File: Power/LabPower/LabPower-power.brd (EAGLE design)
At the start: 97.8 x 128.9 mm, 60 parts, among them IC1 TNY264PN, Q1 STP11NM60ND, Q2 STP11NM60ND, T1 GDT_20X6.5, X1 MKDSN1,5/3-5,08, X2 MKDSN1,5/3-5,08

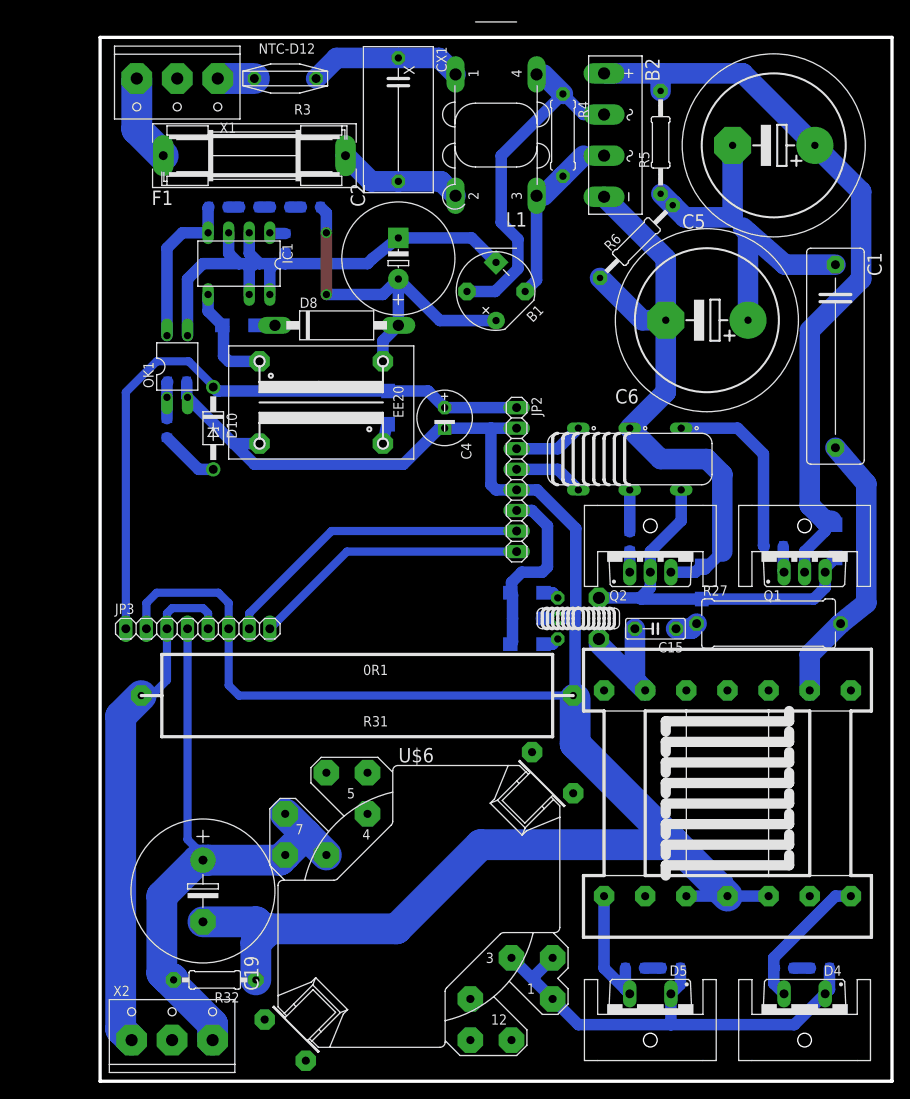
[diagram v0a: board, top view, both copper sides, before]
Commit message: _+
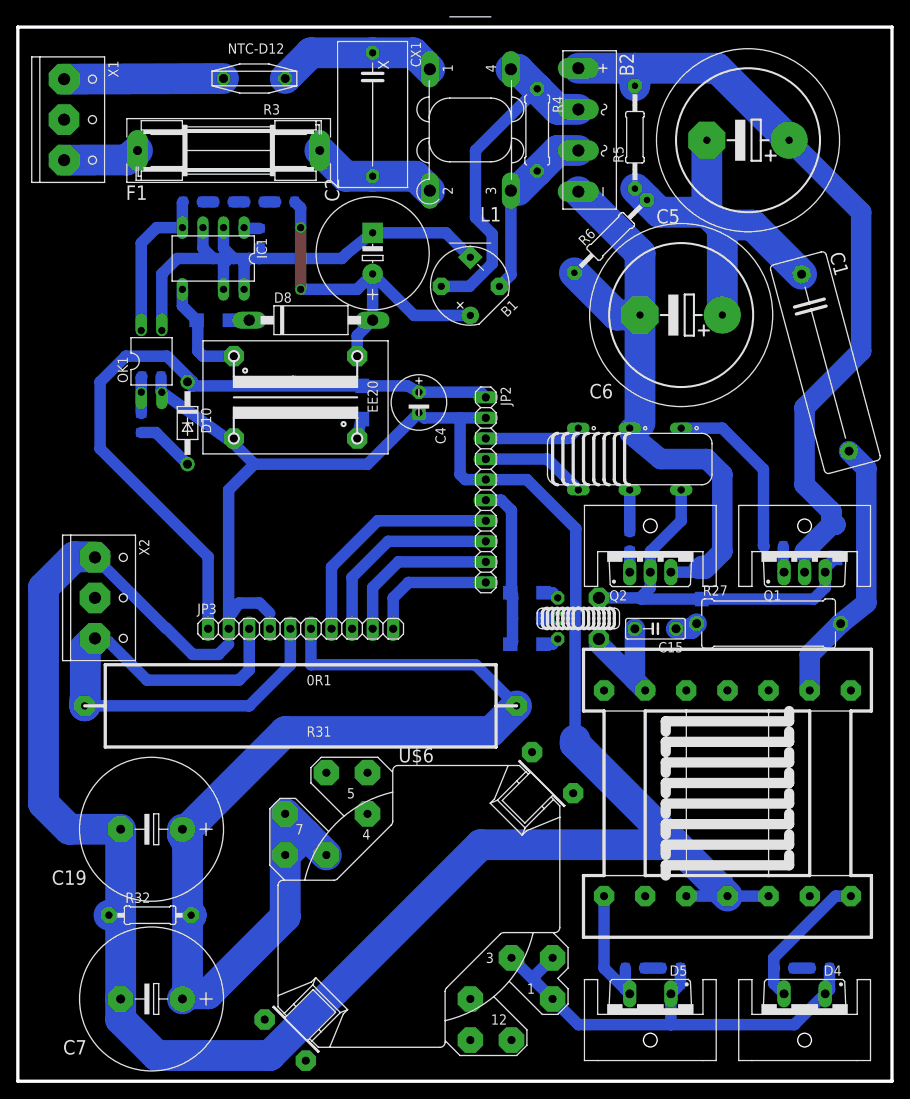
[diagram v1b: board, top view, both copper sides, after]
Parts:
- added C7: 2700u 63V, rcl:E7,5-18
- JP2, JP3: device pinhead:1X08 -> pinhead:1X10
- moved X2 55.4 mm to (-98.4, -69.8), turned to 270 degrees
- moved X1 14.9 mm to (-102.2, -10.8), turned to 270 degrees
- moved JP3 12.7 mm to (-73.0, -73.7)
- moved R32 11.3 mm to (-91.6, -109.0), turned to 0 degrees
- moved C19 9.92 mm to (-91.4, -98.4), turned to 180 degrees
- moved R31 7.10 mm to (-73.0, -83.2)
- moved JP2 4.02 mm to (-50.2, -56.5)
- moved R3 3.81 mm to (-78.7, -5.71)
- moved C4 3.70 mm to (-58.4, -45.7)
- moved D10 3.24 mm to (-87.0, -48.3)
- moved F1 3.24 mm to (-81.9, -14.6)
- moved R12 3.24 mm to (-74.9, -21.0)
- moved C2 3.24 mm to (-64.1, -27.3)
- moved B2 3.24 mm to (-37.5, -12.1)
- moved CX1 3.24 mm to (-64.1, -10.2)
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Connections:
- net I-FB renamed -V-FB
- net V-FB renamed +V-FB
- removed net OUT+: C19.+, JP3.4, R32.2, U$6.7, U$6.8, U$6.9, X2.3
- removed net OUT-/CUR+: JP3.3, JP3.5, R31.P$2, X2.1
- new net +I-FB: JP2.9, JP3.9
- new net -I-FB: JP2.10, JP3.10
- new net CUR+: C19.+, C7.+, JP3.6, R31.P$1, R32.2, U$6.7, U$6.8, U$6.9
- new net OUT+\CUR-: JP3.3, JP3.5, R31.P$2, X2.3
- net GND: now also C7.-, JP3.4, X2.1; no longer JP3.6, R31.P$1
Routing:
- net CUR+: track 0.00 -> 143.2 mm
- net OUT+: track 79.0 -> 0.00 mm
- net GND: track 279.2 -> 348.3 mm
- net OUT+\CUR-: track 0.00 -> 68.5 mm
- net OUT-/CUR+: track 63.9 -> 0.00 mm
- net +I-FB: track 0.00 -> 20.4 mm
- net -I-FB: track 0.00 -> 16.7 mm
- net N$7: track 4.53 -> 19.7 mm
- net +V-FB: track 39.1 -> 29.0 mm
- net -V-FB: track 34.4 -> 24.7 mm
- net +12: track 82.3 -> 88.1 mm
- net N$22: track 8.67 -> 13.0 mm
- net N$18: track 8.67 -> 12.0 mm
- net N$38: track 0.00 -> 2.39 mm
- net 300V: track 92.9 -> 95.2 mm
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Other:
- board size 97.8 x 128.9 mm -> 108 x 130.2 mm
